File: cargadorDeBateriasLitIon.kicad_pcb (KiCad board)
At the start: 2 copper layers, 17 x 12 mm, 13 parts, among them Q1 2N7002, Q2 2N7002, U1 MCP73831-2, U2 AP9101C

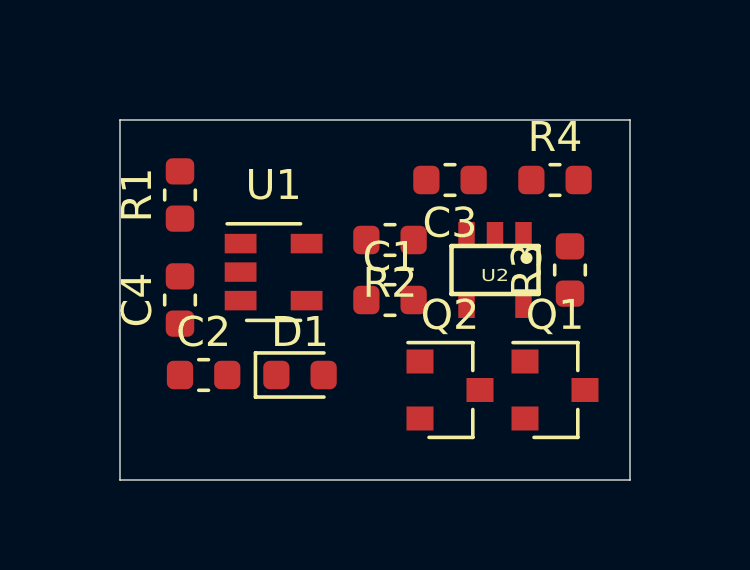
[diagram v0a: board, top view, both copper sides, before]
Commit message: PCB version 1, falta probar
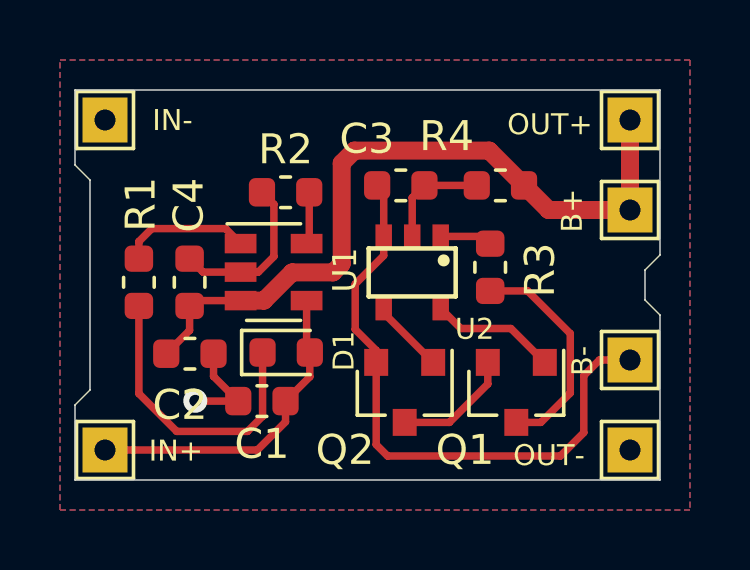
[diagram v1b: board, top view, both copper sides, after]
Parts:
- added G***: LOGO, MSS_Devices:logo-mr_solder_7.8x3.6mm, B.Cu at (149.0, 105.3)
- added J1: IN+, TestPoint:TestPoint_THTPad_1.5x1.5mm_Drill0.7mm, F.Cu at (140.5, 114.0)
- added J2: IN-, TestPoint:TestPoint_THTPad_1.5x1.5mm_Drill0.7mm, F.Cu at (140.5, 103.0)
- added J3: OUT+, TestPoint:TestPoint_THTPad_1.5x1.5mm_Drill0.7mm, F.Cu at (158.0, 106.0)
- added J4: B+, TestPoint:TestPoint_THTPad_1.5x1.5mm_Drill0.7mm, F.Cu at (158.0, 103.0)
- added J5: B-, TestPoint:TestPoint_THTPad_1.5x1.5mm_Drill0.7mm, F.Cu at (158.0, 111.0)
- added J6: OUT-, TestPoint:TestPoint_THTPad_1.5x1.5mm_Drill0.7mm, F.Cu at (158.0, 114.0)
- moved C1 5.44 mm to (145.7, 112.4), turned to 180 degrees
- moved R2 3.83 mm to (146.5, 105.4), turned to 0 degrees
- moved R1 3.22 mm to (141.6, 108.4), turned to 270 degrees
- moved U2 2.76 mm to (150.7, 108.1)
- moved R3 2.66 mm to (153.3, 107.9)
- moved R4 1.83 mm to (153.7, 105.2)
- moved C3 1.65 mm to (150.4, 105.2)
- moved Q2 1.51 mm to (150.5, 112.1), turned to 270 degrees
- moved Q1 1.29 mm to (154.2, 112.1), turned to 270 degrees
- moved D1 0.88 mm to (146.5, 110.8)
- moved C2 0.84 mm to (143.3, 110.8)
- moved C4 0.67 mm to (143.3, 108.4)
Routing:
- net /B+: track 0.00 -> 24.5 mm
- net /B-: track 0.00 -> 20.5 mm
- net /IN+: track 0.00 -> 10.8 mm
- net Net-(D1-Pad1): track 0.00 -> 9.90 mm
- net GND: track 0.00 -> 8.87 mm, vias 0 -> 1
- net Net-(Q1-Pad3): track 0.00 -> 7.45 mm
- net Net-(R1-Pad1): track 0.00 -> 4.35 mm
- net Net-(Q1-Pad1): track 0.00 -> 4.22 mm
- net Net-(Q1-Pad2): track 0.00 -> 4.02 mm
- net Net-(C3-Pad1): track 0.00 -> 3.61 mm
- net Net-(Q2-Pad1): track 0.00 -> 2.48 mm
- net Net-(R3-Pad2): track 0.00 -> 1.75 mm
- net Net-(R2-Pad2): track 0.00 -> 1.75 mm
- added copper zone on B.Cu, net GND
- added copper zone on F.Cu, net GND
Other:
- board size 17 x 12 mm -> 19.5 x 13 mm
- board text added: "B+"
- board text added: "B-"
- board text added: "IN+"
- board text added: "IN-"
- board text added: "OUT+"
- board text added: "OUT-"
